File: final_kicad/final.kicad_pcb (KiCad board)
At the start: 2 copper layers, 10 x 95.5 mm, 19 parts, among them J1 Signal, J2 Battery, J3 Power, M1 Motor_DC, Q1 NPN, SW1 SW_SPST, SW2 SW_Push, U1 MPU-6050

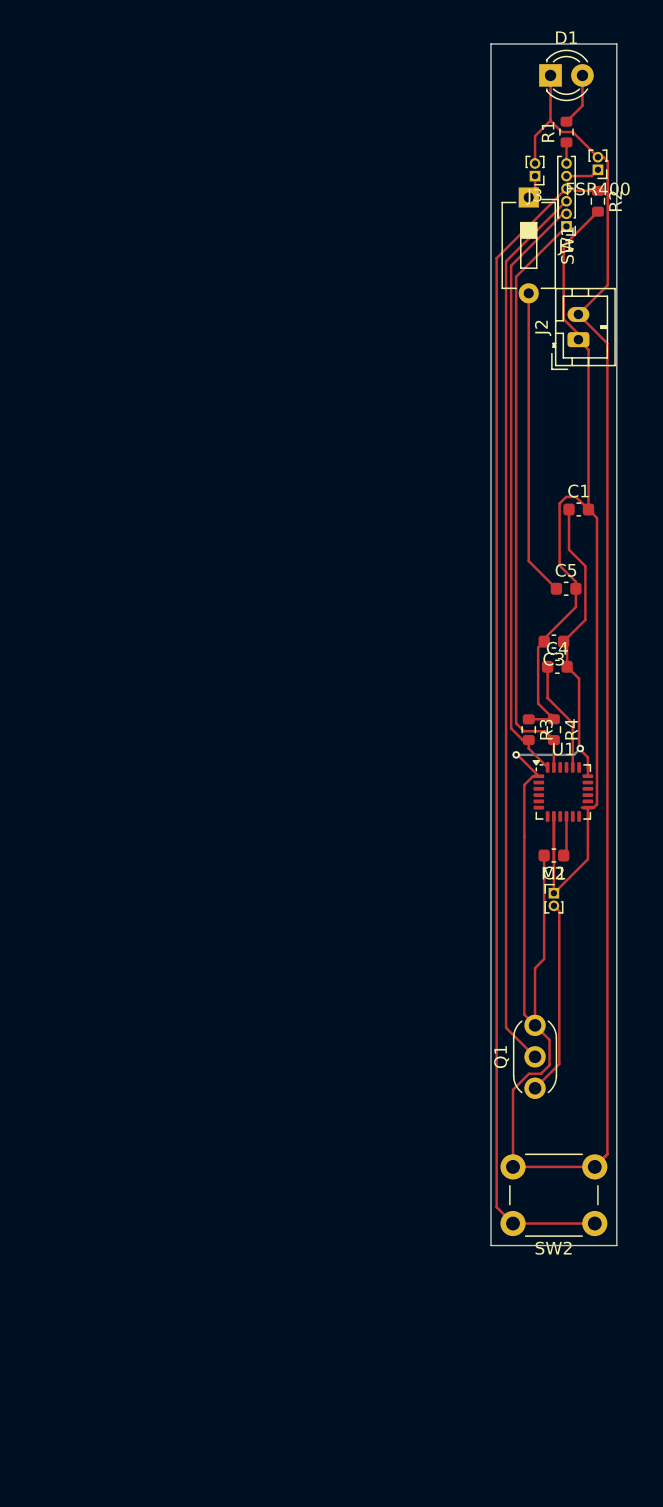
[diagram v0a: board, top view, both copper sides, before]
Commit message: 1
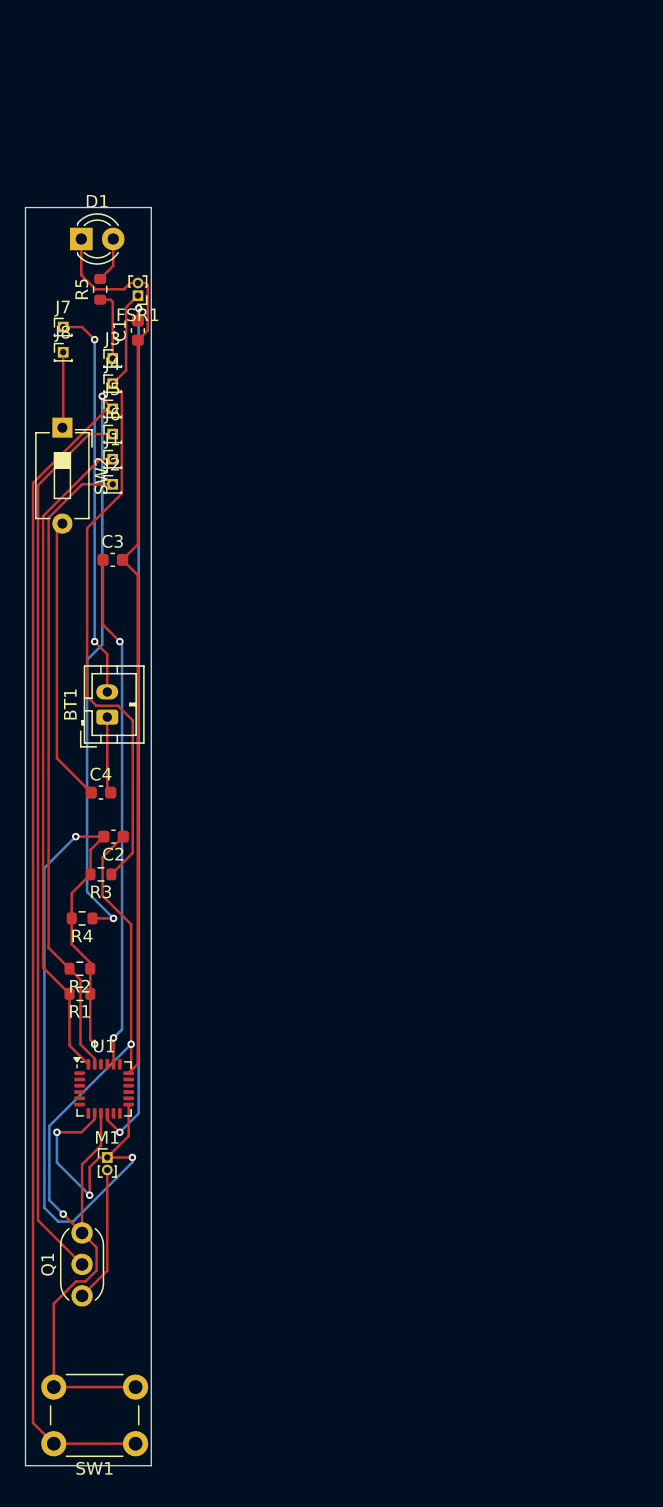
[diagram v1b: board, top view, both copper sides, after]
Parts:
- removed C5: 10uF, Capacitor_SMD:C_0603_1608Metric
- removed FSR400: 10K, Connector_PinHeader_1.00mm:PinHeader_1x02_P1.00mm_Vertical
- added BT1: Battery_Cell, Connector_JST:JST_PH_B2B-PH-K_1x02_P2.00mm_Vertical, F.Cu at (119.5, 74.0)
- added FSR1: 10K, Connector_PinHeader_1.00mm:PinHeader_1x02_P1.00mm_Vertical, F.Cu at (121.9, 40.5)
- added J4: PIN2, Connector_PinHeader_1.00mm:PinHeader_1x01_P1.00mm_Vertical, F.Cu at (119.9, 47.5)
- added J5: PIN3, Connector_PinHeader_1.00mm:PinHeader_1x01_P1.00mm_Vertical, F.Cu at (119.9, 49.5)
- added J6: PIN4, Connector_PinHeader_1.00mm:PinHeader_1x01_P1.00mm_Vertical, F.Cu at (119.9, 51.5)
- added J7: neg, Connector_PinHeader_1.00mm:PinHeader_1x01_P1.00mm_Vertical, F.Cu at (116.0, 43.0)
- added J8: pos, Connector_PinHeader_1.00mm:PinHeader_1x01_P1.00mm_Vertical, F.Cu at (116.0, 45.0)
- added R5: 200, Resistor_SMD:R_0603_1608Metric, F.Cu at (118.9, 40.0)
- C3: value 0.1U -> 2200PF
- C4: value 2200PF -> 10uF
- J1: value Signal -> SDA; footprint Connector_PinHeader_1.00mm:PinHeader_1x06_P1.00mm_Vertical -> Connector_PinHeader_1.00mm:PinHeader_1x01_P1.00mm_Vertical
- J2: value Battery -> SCL; footprint Connector_JST:JST_PH_B2B-PH-K_1x02_P2.00mm_Vertical -> Connector_PinHeader_1.00mm:PinHeader_1x01_P1.00mm_Vertical
- J3: value Power -> PIN1; footprint Connector_PinHeader_1.00mm:PinHeader_1x02_P1.00mm_Vertical -> Connector_PinHeader_1.00mm:PinHeader_1x01_P1.00mm_Vertical
- R1: value 200 -> 4.7K
- R2: value 10k -> 4.7K
- R3, R4: value 4.7K -> 10k
- SW1: value SW_SPST -> SW_Push; footprint Button_Switch_THT:SW_DIP_SPSTx01_Slide_6.7x4.1mm_W7.62mm_P2.54mm_LowProfile -> Button_Switch_THT:SW_PUSH_6mm
- SW2: value SW_Push -> SW_SPST; footprint Button_Switch_THT:SW_PUSH_6mm -> Button_Switch_THT:SW_DIP_SPSTx01_Slide_6.7x4.1mm_W7.62mm_P2.54mm_LowProfile
- moved SW1 103.9 mm to (121.8, 131.8), turned to 180 degrees
- moved R1 78.7 mm to (117.3, 96.0), turned to 180 degrees
- moved SW2 76.1 mm to (115.9, 51.0), turned to -90 degrees
- moved R2 73.6 mm to (117.3, 94.0), turned to 180 degrees
- moved U1 43.5 mm to (119.2, 103.5)
- moved M1 41.2 mm to (119.5, 109.0)
- moved J1 40.5 mm to (119.9, 53.5), turned to 0 degrees
- moved R4 40.4 mm to (117.5, 90.0), turned to 180 degrees
- moved Q1 39.6 mm to (117.5, 120.0)
- moved D1 39.5 mm to (117.4, 36.0)
- moved J2 38.8 mm to (119.9, 55.5), turned to 0 degrees
- moved C1 37.8 mm to (121.9, 43.3), turned to 90 degrees
- moved C4 37.6 mm to (119.0, 80.0)
- moved J3 36.6 mm to (119.9, 45.5), turned to 0 degrees
- moved R3 35.9 mm to (119.0, 86.5), turned to 180 degrees
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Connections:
- C1 pad 1: Net-(D1-K) -> GND
- C1 pad 2: Net-(J2-Pin_1) -> Net-(U1-REGOUT)
- C2 pad 1: Net-(U1-REGOUT) -> GND
- C2 pad 2: Net-(D1-K) -> +3V3
- C3 pad 1: Net-(D1-K) -> Net-(U1-CPOUT)
- C3 pad 2: Net-(J2-Pin_1) -> GND
- C4 pad 1: Net-(U1-CPOUT) -> Net-(SW2-B)
- C4 pad 2: Net-(D1-K) -> Net-(BT1-+)
- D1 pad 1: Net-(D1-K) -> GND
- M1 pad 1: Net-(J2-Pin_1) -> +3V3
- Q1 pad 2: Net-(J1-Pin_3) -> Net-(J6-Pin_1)
- Q1 pad 3: Net-(D1-K) -> GND
- R1 pad 1: Net-(J1-Pin_6) -> +3V3
- R1 pad 2: Net-(D1-A) -> Net-(J1-Pin_1)
- R2 pad 1: Net-(J1-Pin_4) -> +3V3
- R3 pad 1: Net-(J2-Pin_1) -> Net-(J4-Pin_1)
- R3 pad 2: Net-(J1-Pin_2) -> +3V3
- R4 pad 1: Net-(J2-Pin_1) -> Net-(J5-Pin_1)
- R4 pad 2: Net-(J1-Pin_1) -> +3V3
- SW1 pad 1: Net-(J3-Pin_1) -> Net-(J5-Pin_1)
- SW1 pad 2: Net-(SW1-B) -> GND
- SW2 pad 1: Net-(J1-Pin_4) -> Net-(J8-Pin_1)
- SW2 pad 2: Net-(D1-K) -> Net-(SW2-B)
- U1 pad 1: Net-(D1-K) -> unconnected-(U1-CLKIN-Pad1)
- U1 pad 13: Net-(J2-Pin_1) -> +3V3
- U1 pad 18: Net-(D1-K) -> GND
- U1 pad 23: Net-(J1-Pin_1) -> Net-(J2-Pin_1)
- U1 pad 24: Net-(J1-Pin_2) -> Net-(J1-Pin_1)
- U1 pad 8: Net-(J2-Pin_1) -> +3V3
- U1 pad 9: unconnected-(U1-AD0-Pad9) -> GND
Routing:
- net Net-(D1-K): track 183.2 -> 0.00 mm, vias 2 -> 0
- net GND: track 0.00 -> 143.6 mm, vias 0 -> 2
- net Net-(J5-Pin_1): track 0.00 -> 138.2 mm, vias 0 -> 2
- net Net-(J1-Pin_4): track 94.2 -> 0.00 mm
- net +3V3: track 0.00 -> 81.7 mm, vias 0 -> 5
- net Net-(J1-Pin_3): track 71.1 -> 0.00 mm
- net Net-(J6-Pin_1): track 0.00 -> 71.0 mm
- net Net-(U1-REGOUT): track 3.19 -> 69.1 mm, vias 0 -> 2
- net Net-(J4-Pin_1): track 0.00 -> 51.5 mm
- net Net-(J1-Pin_2): track 47.5 -> 0.00 mm
- net Net-(J2-Pin_1): track 92.9 -> 51.2 mm
- net Net-(U1-CPOUT): track 8.84 -> 41.0 mm, vias 0 -> 2
- net Net-(BT1--): track 0.00 -> 31.3 mm, vias 0 -> 2
- net Net-(SW1-B): track 24.4 -> 0.00 mm
- net Net-(SW2-B): track 0.00 -> 22.3 mm
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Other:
- board size 10 x 95.5 mm -> 10 x 100 mm
